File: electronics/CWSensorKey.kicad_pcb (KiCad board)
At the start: 2 copper layers, 37 x 30 mm, 21 parts, among them J1 Tip, J2 GND, J3 Ring, J4 Dit, J5 Dah, J6 +, J7 -, Q1 IRFML8244TRPBF, Q2 IRFML8244TRPBF, U1 AT42QT1011, U2 AT42QT1011

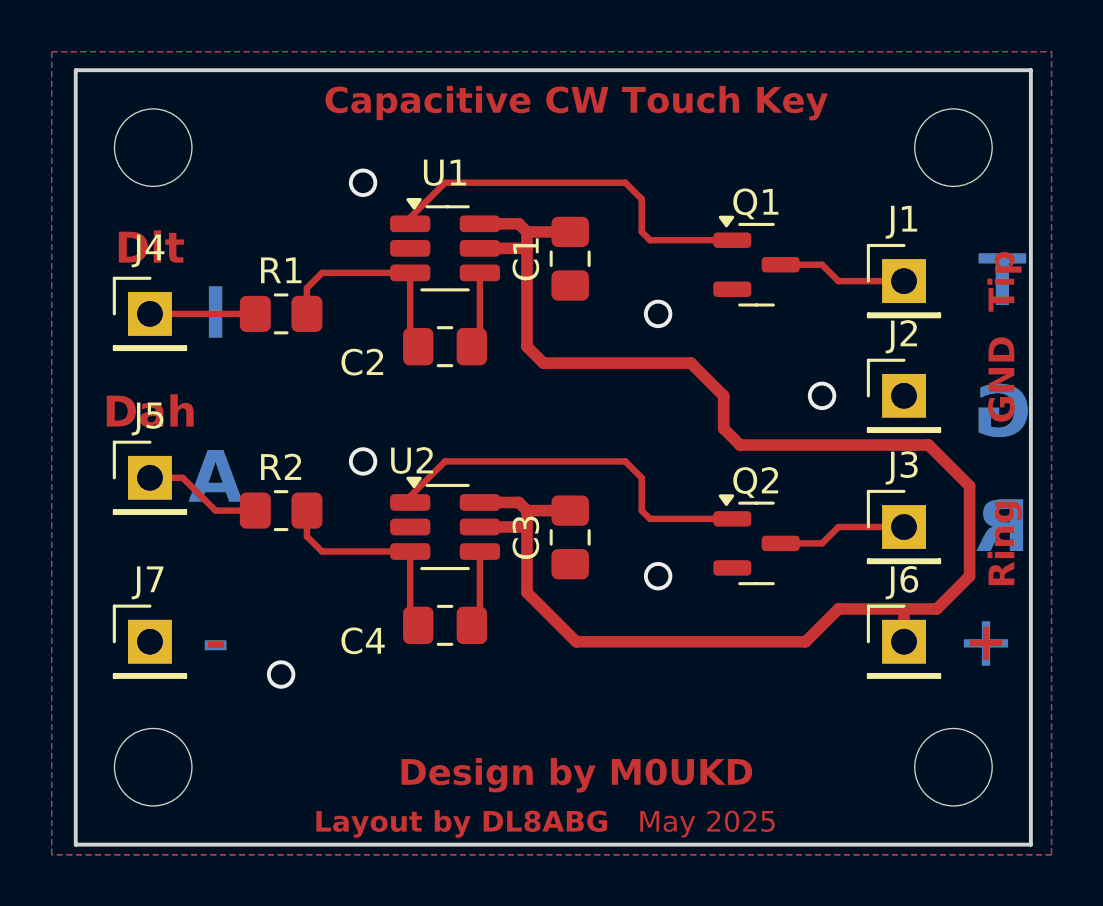
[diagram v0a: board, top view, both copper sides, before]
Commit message: Branch (#3)
* index on main: b7a867d Further documentation in README.md Slightly changed dimensions of sensor pad Changed distance betw screws in sensor pad holder

* Adapted board for better fitting in the housing
Implemented script for generation of all 2D files from the KiCad models

* Delete electronics/gerbers directory

resolving merge conflict

* Update CWSensorKey.kicad_prl

updated active layer in kicad project file

---------

Co-authored-by: DL8ABG <dl8abg@qsl.net>
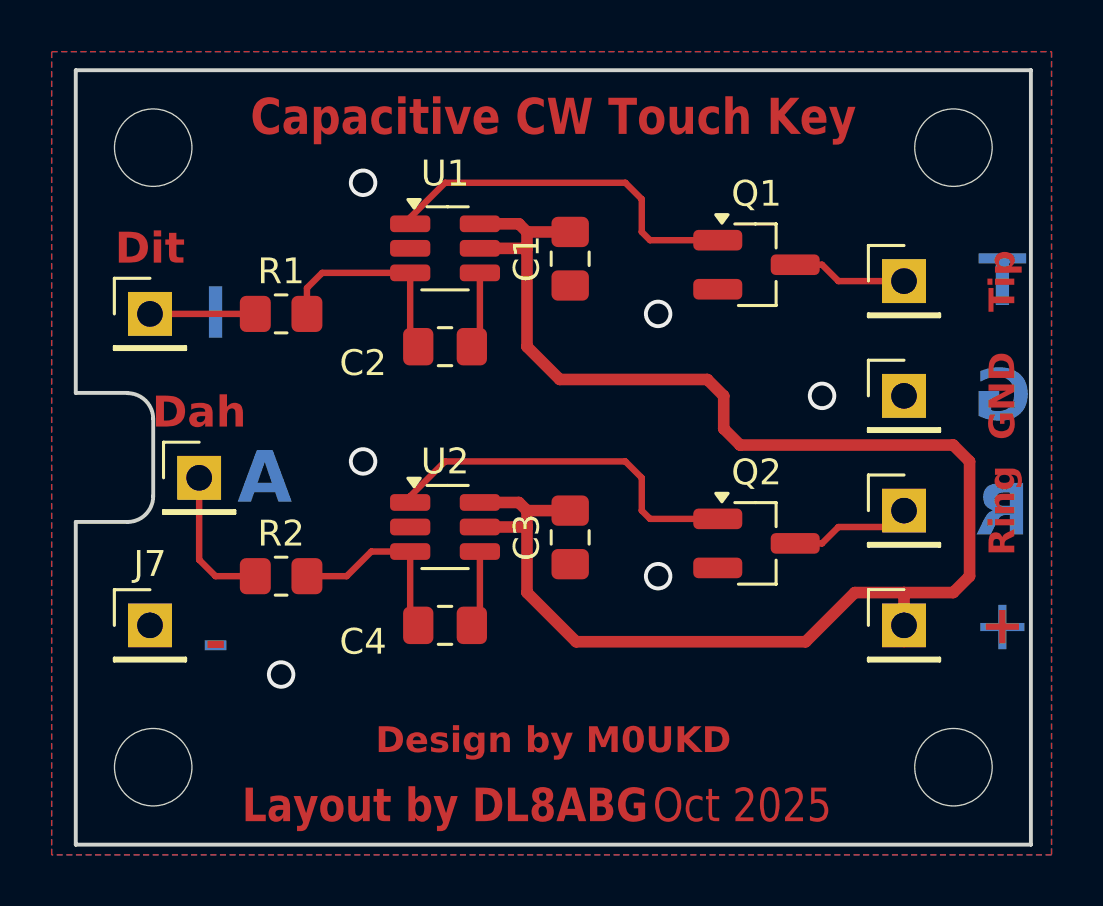
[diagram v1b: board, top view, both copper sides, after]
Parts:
- H1, H2, H3, H4: footprint MountingHole:MountingHole_2.7mm_M2.5_DIN965 -> MountingHole:MountingHole_3mm
- Q1, Q2: footprint Package_TO_SOT_SMD:SOT-23 -> Package_TO_SOT_SMD:SOT-23_Handsoldering
- moved R2 2.54 mm to (148.0, 101.6)
- moved J5 1.91 mm to (144.8, 97.8)
- moved J6 0.64 mm to (172.1, 103.5)
- moved J7 0.64 mm to (142.9, 103.5)
- moved J3 0.63 mm to (172.1, 99.1)
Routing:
- net +3.3V: track 62.5 -> 63.7 mm
- net Net-(J5-Pin_1): track 4.61 -> 5.61 mm
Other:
- outline, holes or cut-outs redrawn
- board text added: "Oct 2025"
- board text removed: "May 2025"
